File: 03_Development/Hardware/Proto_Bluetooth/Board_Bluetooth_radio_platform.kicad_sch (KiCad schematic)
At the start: 47 parts, among them J1 Conn_01x02, J10 Conn_01x03, J11 HMI_rotaryEncoder_1, J12 HMI_rotaryEncoder_1, J19 Conn_01x02_rn52_usb, J2 Conn_01x08, J3 BT_RN52_connector_left, J4 Conn_01x02, J5 BT_RN52_connector_right, J6 FM_interface, J7 BT_debug_connector, J8 BT_extension_connector, J9 SYS_debug_connector, SW1 SW_Push, U1 LM317_TO-220

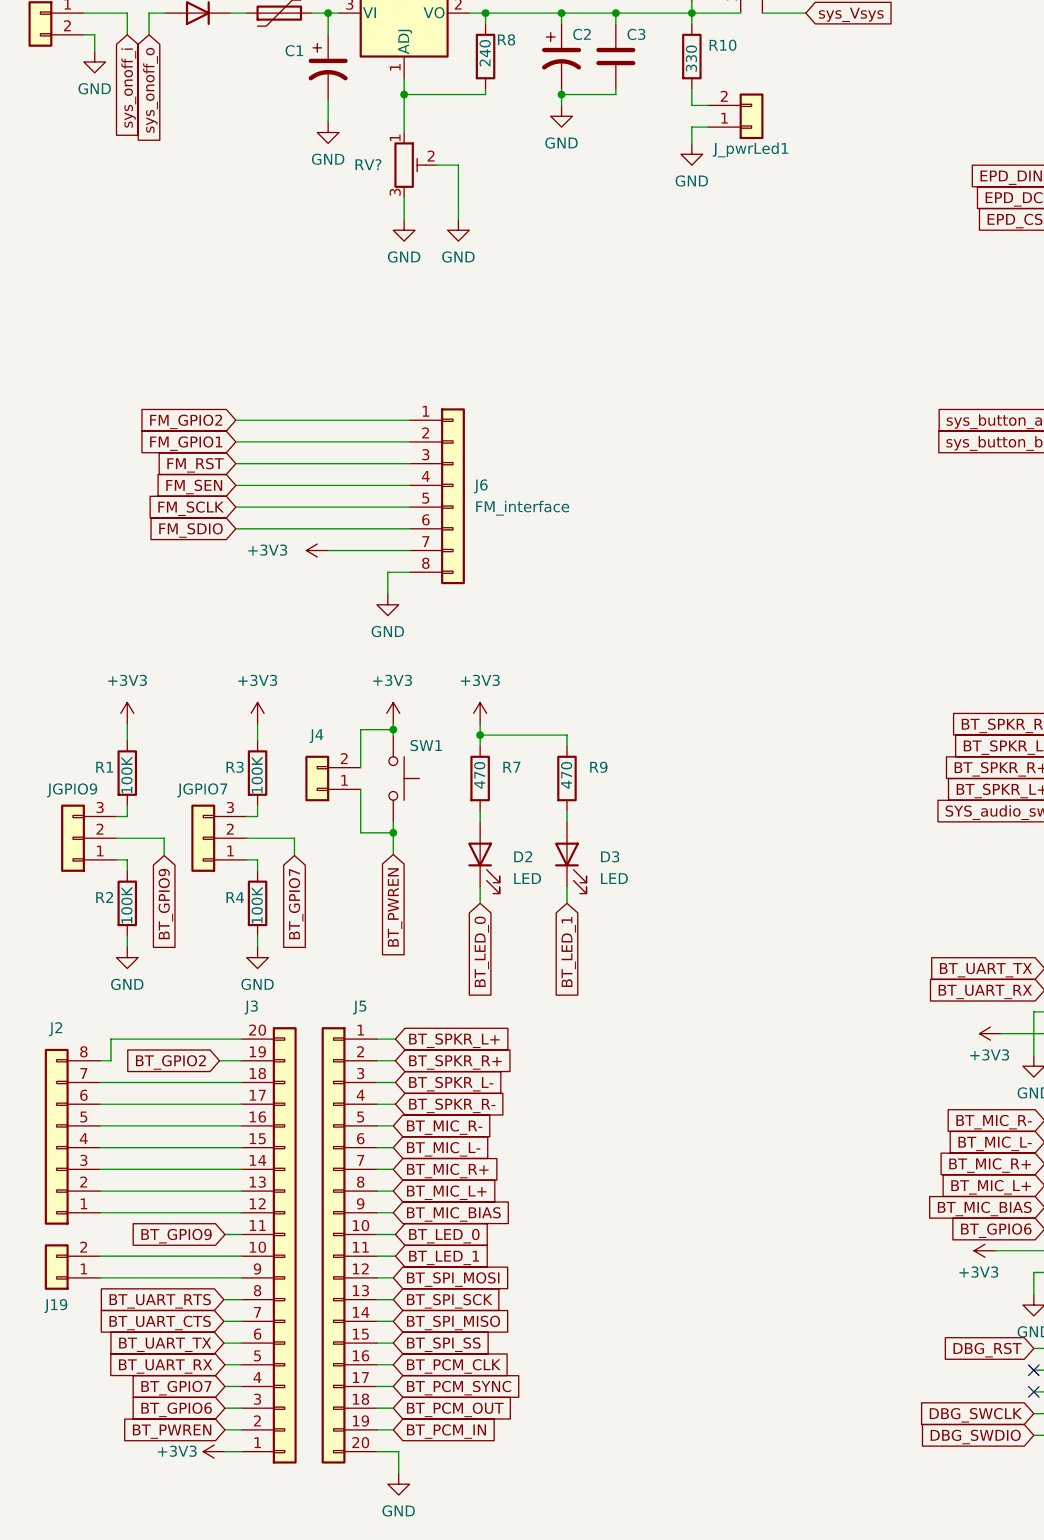
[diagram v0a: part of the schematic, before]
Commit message: [HDW_31] Add 1205V DC DC converter
Add of a murata NXE2S1205MC DC DC downconverter
to add 12V power supply possibility. Will maybe
not be soldered but footprints are there for
future amelioration. Helps to plug a battery
on radio
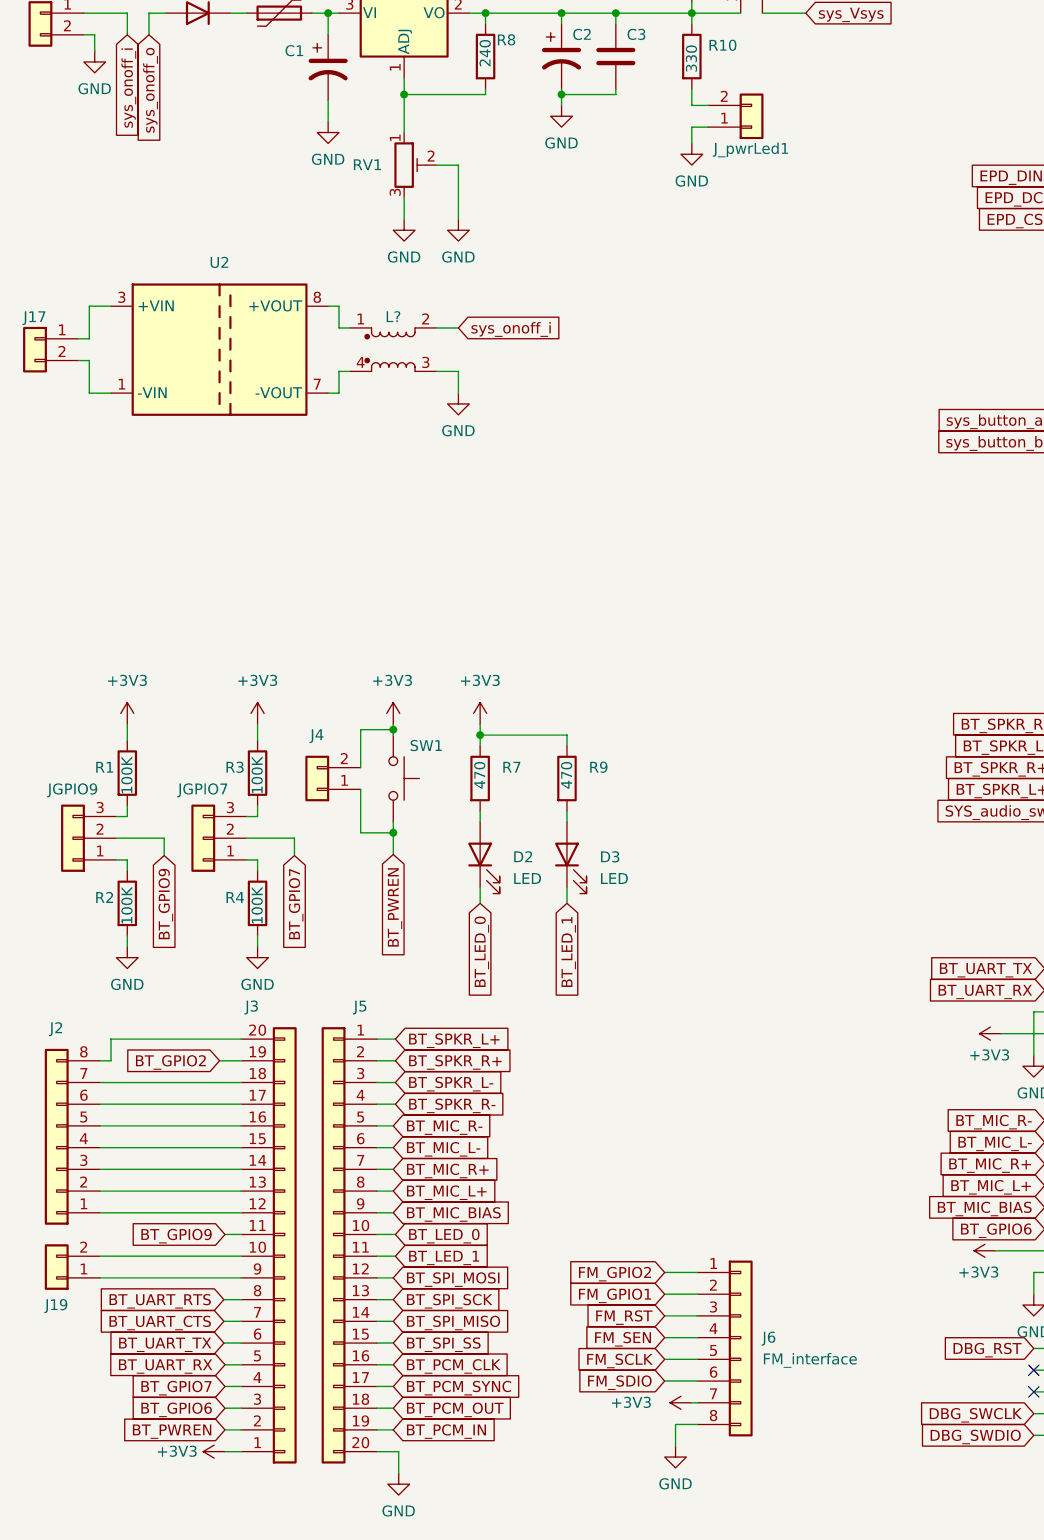
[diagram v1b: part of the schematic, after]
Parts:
- added J17: Conn_01x02, Connector_PinSocket_2.54mm:PinSocket_1x02_P2.54mm_Vertical, symbol Connector_Generic:Conn_01x02
- added L?: L_Coupled_1243 22n, Inductor_SMD:L_Wuerth_WE-DD-Typ-M-Typ-S, symbol Device:L_Coupled_1243
- added U2: NXE2S1205MC, Converter_DCDC:Converter_DCDC_Murata_NXExSxxxxMC_SMD, symbol Regulator_Switching:NXE2S1205MC
- gave numbers to parts that had none: 1
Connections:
- net GND: now also L?.3
- net sys_onoff_i: now also L?.2
- new net: L?.1, U2.8 (+VOUT)
- new net: L?.4, U2.7 (-VOUT)
- new net: J17.1 (Pin_1), U2.3 (+VIN)
- new net: J17.2 (Pin_2), U2.1 (-VIN)
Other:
- moved on the sheet: J6

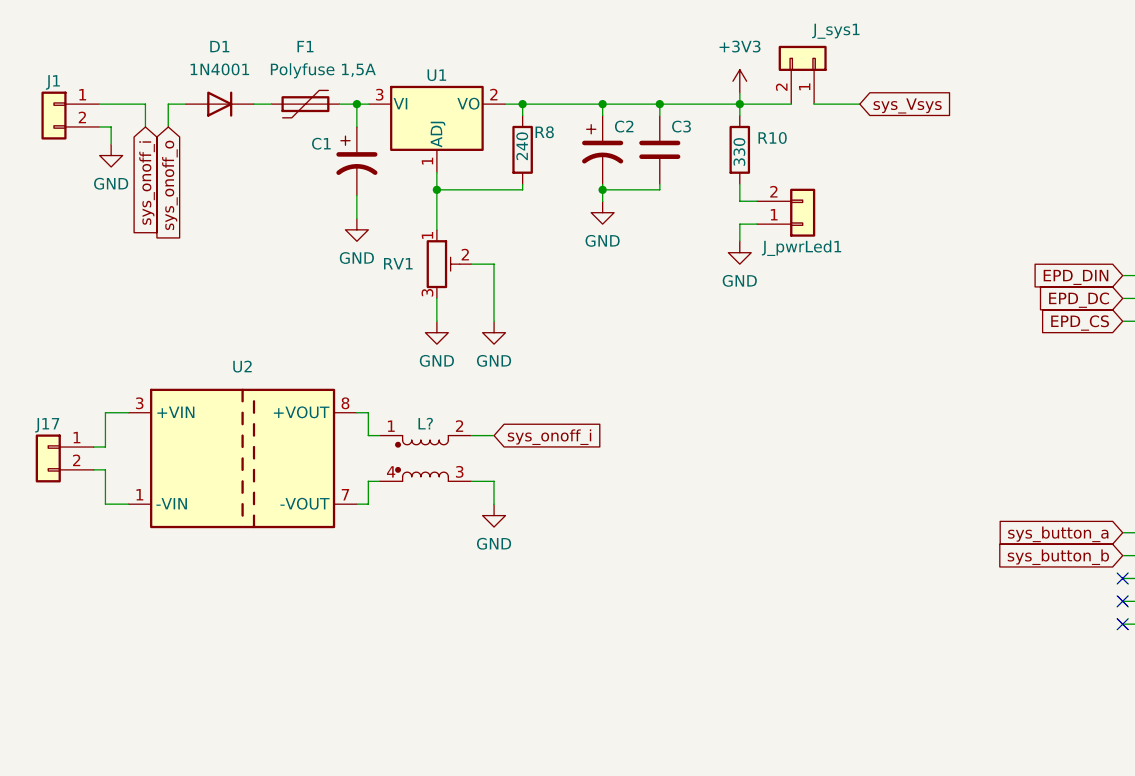
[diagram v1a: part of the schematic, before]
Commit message: [HDW_36] Fixed edge cut layer
Edge.cut layer fixed with circle removed
Cleanup TICKET.md file
minor other correction
READY TO TEST. All firmware should be tested
on breadboard first before sending to production
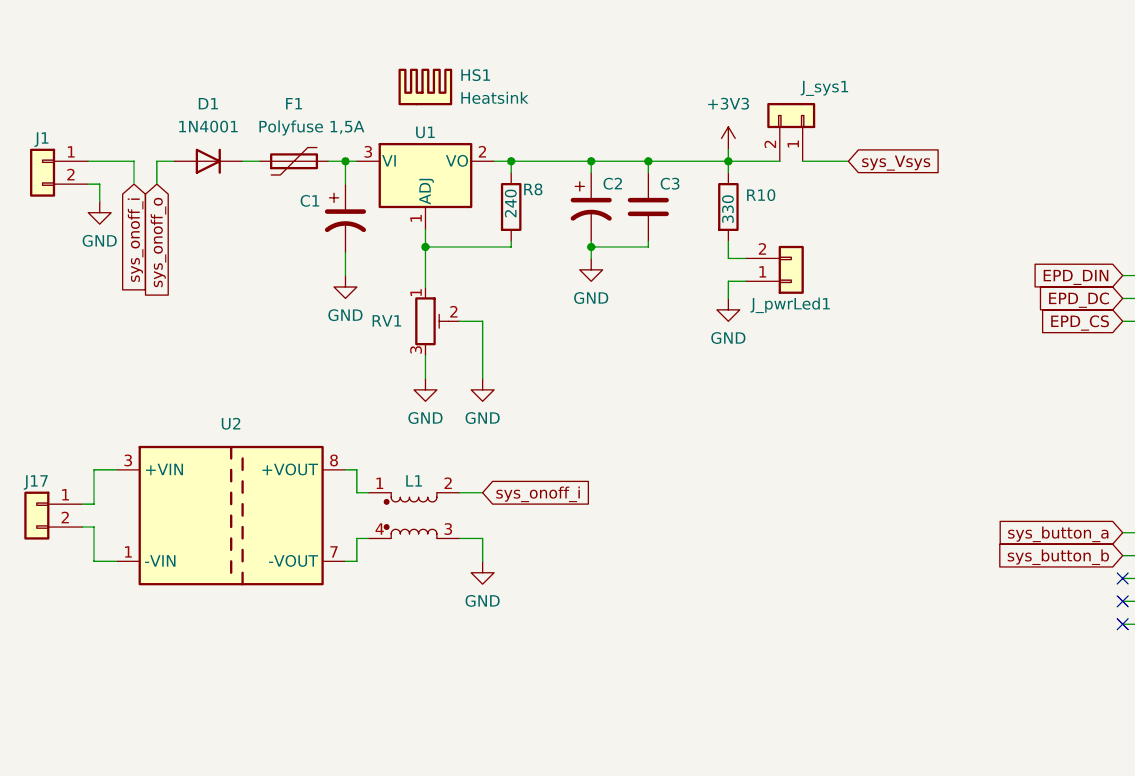
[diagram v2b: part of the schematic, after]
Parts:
- added HS1: Heatsink, Heatsink:Heatsink_AAVID_TV5G_TO220_Horizontal, symbol Mechanical:Heatsink
- L1: renamed from L?; Mouser (none) -> 710-744877220
- RV1: Mouser (none) -> 652-3299W-1-102LF
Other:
- moved on the sheet: C1, C2, C3, D1, F1, J1, J17, J_pwrLed1, J_sys1, L1, R10, R8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

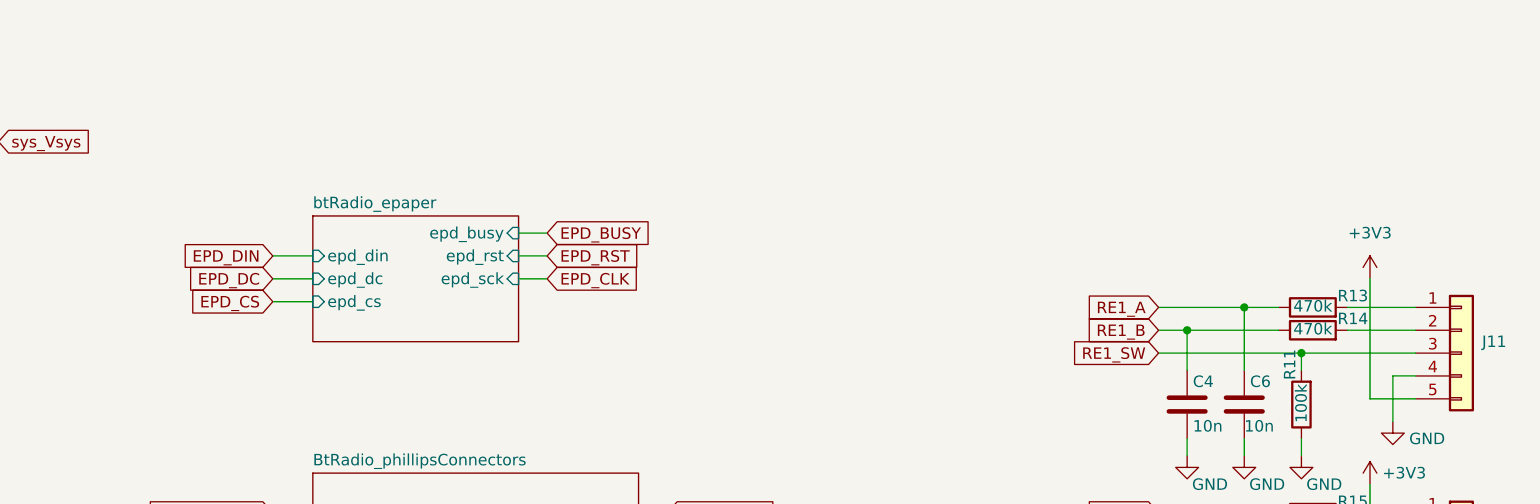
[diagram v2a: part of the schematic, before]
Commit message: Add pictures and remove epaper connector in schematics
Schematic of epaper was pointless as alone in its file. Moved to main schematic
Add pictures of schematic and PCB for documentation
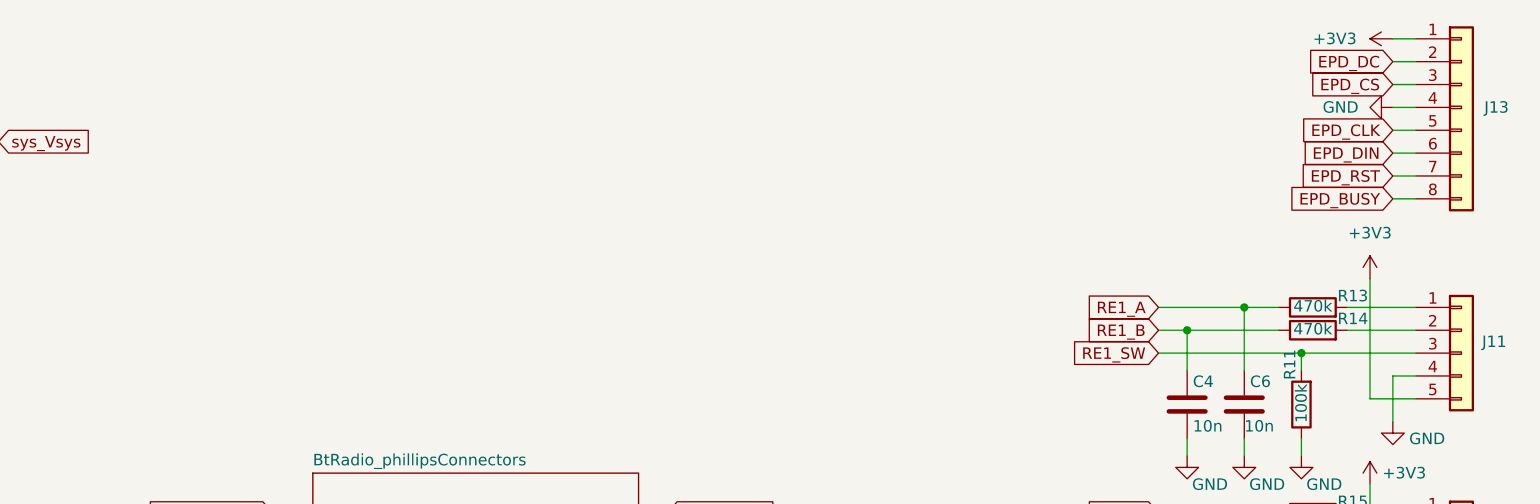
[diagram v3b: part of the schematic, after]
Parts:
- added J13: Conn_01x08_epaper, Connector_PinSocket_2.54mm:PinSocket_1x08_P2.54mm_Vertical, symbol Connector_Generic:Conn_01x08
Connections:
- net +3V3: now also J13.1 (Pin_1)
- net EPD_BUSY: now also J13.8 (Pin_8)
- net EPD_CLK: now also J13.5 (Pin_5)
- net EPD_CS: now also J13.3 (Pin_3)
- net EPD_DC: now also J13.2 (Pin_2)
- net EPD_DIN: now also J13.6 (Pin_6)
- net EPD_RST: now also J13.7 (Pin_7)
- net GND: now also J13.4 (Pin_4)
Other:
- removed sheet btRadio_epaper
